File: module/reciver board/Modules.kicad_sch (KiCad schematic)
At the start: 25 parts, among them U10 LTC4316xDD, U13 OSMC Module Board, U14 OSMC Module Board, U15 OSMC Module Board, U16 OSMC Module Board, U17 OSMC Module Board, U18 OSMC Module Board, U19 OSMC Module Board, U20 OSMC Module Board, U5 LTC4316xDD, U6 LTC4317

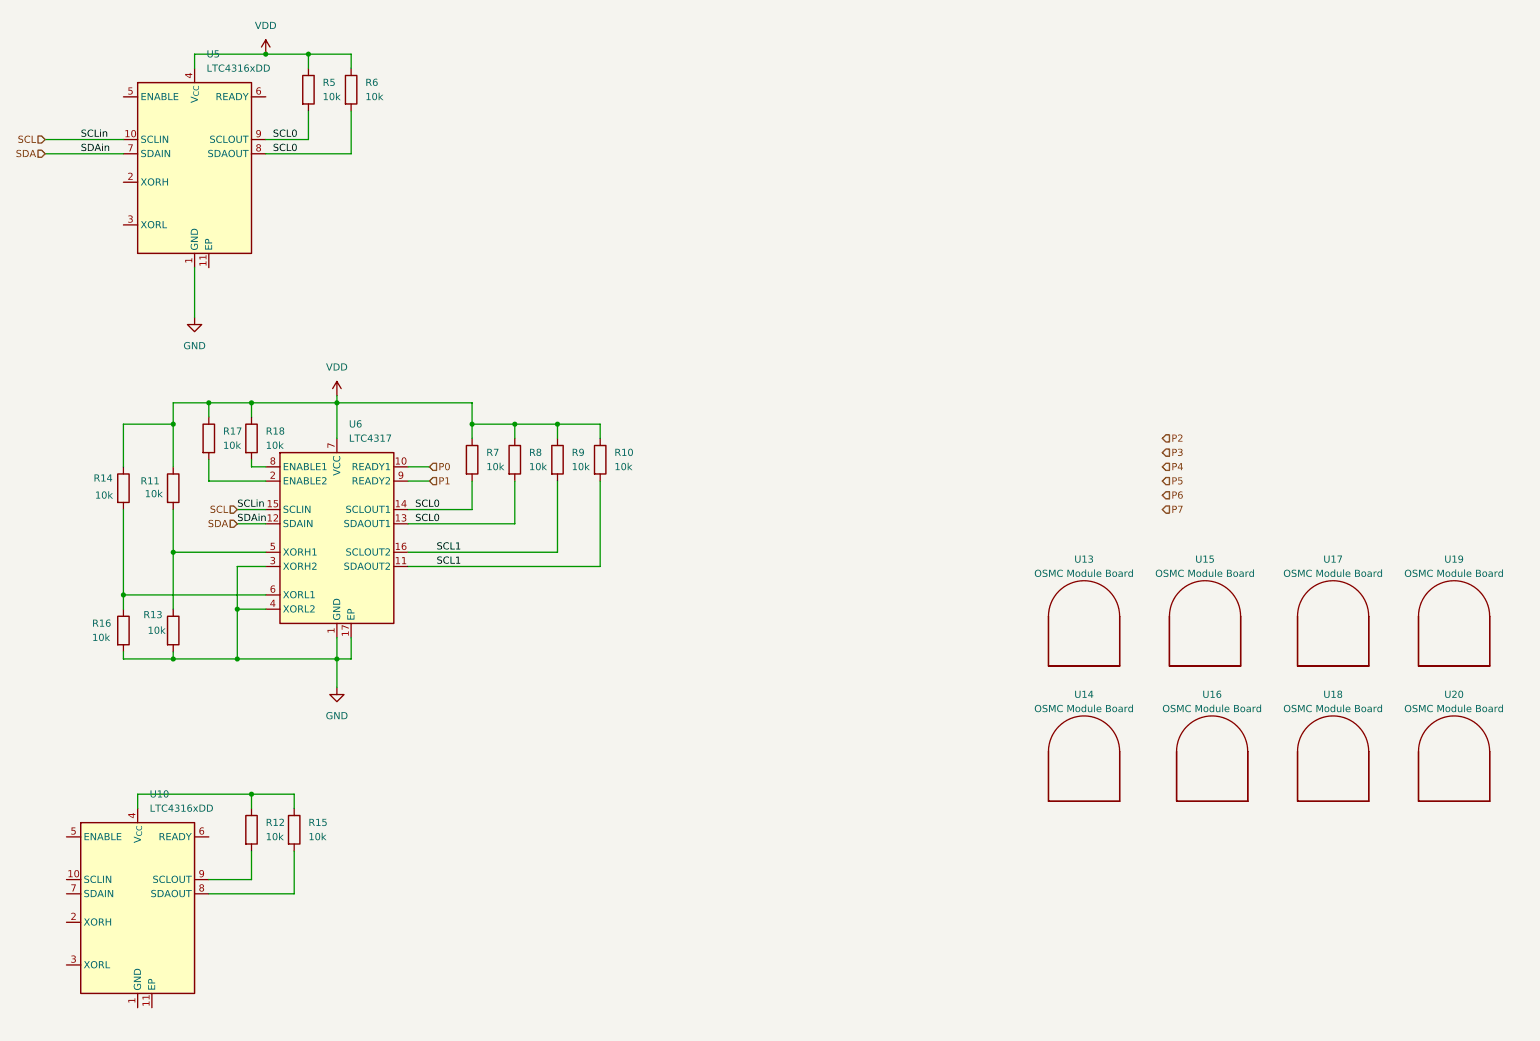
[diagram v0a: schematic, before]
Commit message: update
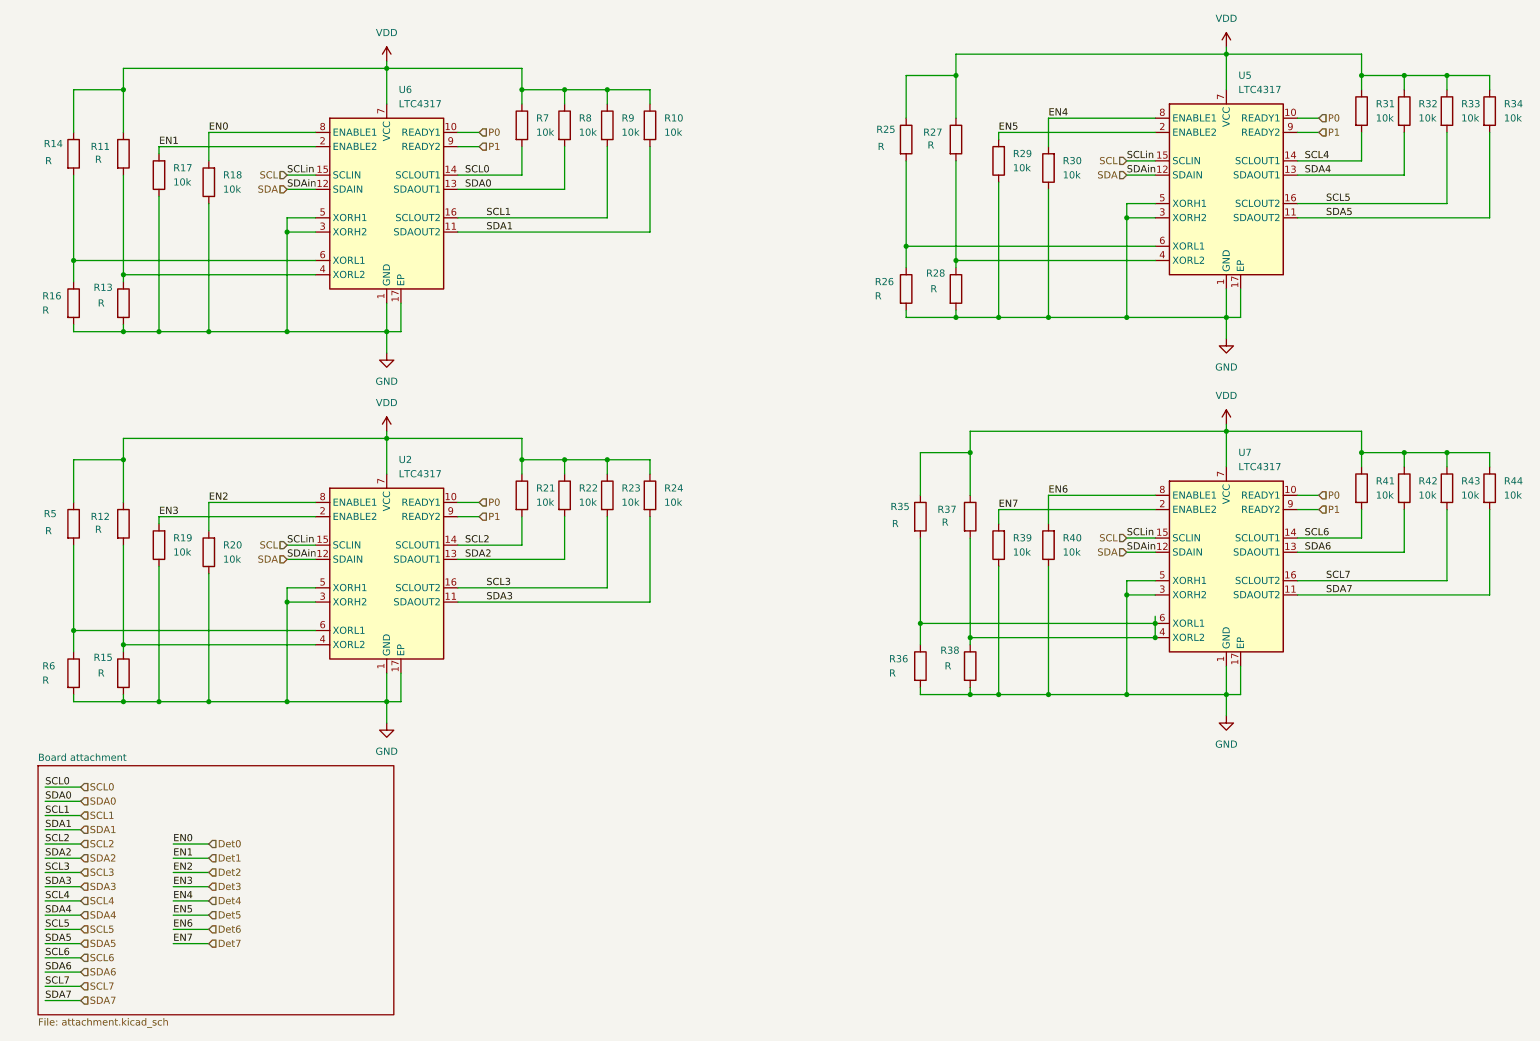
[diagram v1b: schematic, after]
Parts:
- removed U10, U5: LTC4316xDD, Package_DFN_QFN:DFN-10-1EP_3x3mm_P0.5mm_EP1.65x2.38mm, symbol Library:LTC4316xDD
- removed U13, U14, U15, U16, U17, U18, U19, U20: OSMC Module Board, OSMC_Module:Module standard large, symbol Library:Input_Module_Pinless
- added R19, R20, R21, R22, R23, R24, R29, R30, R31, R32, R33, R34, R39, R40, R41, R42, R43, R44: 10k, PCM_Resistor_SMD_AKL:R_0603_1608Metric_Pad1.05x0.95mm_HandSolder, symbol Library:R
- added R25, R26, R27, R28, R35, R36, R37, R38: R, PCM_Resistor_SMD_AKL:R_0603_1608Metric_Pad1.05x0.95mm_HandSolder, symbol Library:R
- added U2, U5, U7: LTC4317, Package_DFN_QFN:DFN-16-1EP_3x5mm_P0.5mm_EP1.66x4.4mm, symbol Library:LTC4317
- R10, R17, R18, R7, R8, R9: footprint PCM_Resistor_SMD_AKL:R_0805_2012Metric_Pad1.15x1.40mm_HandSolder -> PCM_Resistor_SMD_AKL:R_0603_1608Metric_Pad1.05x0.95mm_HandSolder
- R11, R12, R13, R14, R15, R16, R5, R6: value 10k -> R; footprint PCM_Resistor_SMD_AKL:R_0805_2012Metric_Pad1.15x1.40mm_HandSolder -> PCM_Resistor_SMD_AKL:R_0603_1608Metric_Pad1.05x0.95mm_HandSolder
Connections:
- net GND: now also R15.2, R17.1, R18.1, R6.2, U6.5 (XORH1), R19.1, R20.1, R26.2, R28.2, R29.1, R30.1, R36.2, R38.2, R39.1, R40.1, U2.1 (GND), U2.17 (EP), U2.3 (XORH2), U2.5 (XORH1), U5.1 (GND), U5.17 (EP), U5.3 (XORH2), U5.5 (XORH1), U7.1 (GND), U7.17 (EP), U7.3 (XORH2), U7.5 (XORH1); no longer U6.4 (XORL2)
- net P0: now also U2.10 (READY1), U5.10 (READY1), U7.10 (READY1)
- net P1: now also U2.9 (READY2), U5.9 (READY2), U7.9 (READY2)
- net SCL: now also U2.15 (SCLIN), U5.15 (SCLIN), U7.15 (SCLIN)
- net SCL0: no longer R5.2, R6.2, R8.2, U6.13 (SDAOUT1)
- net SCL1: no longer R10.2, U6.11 (SDAOUT2)
- net SDA: now also U2.12 (SDAIN), U5.12 (SDAIN), U7.12 (SDAIN)
- net VDD: now also R12.1, R21.1, R22.1, R23.1, R24.1, R25.1, R27.1, R31.1, R32.1, R33.1, R34.1, R35.1, R37.1, R41.1, R42.1, R43.1, R44.1, U2.7 (VCC), U5.7 (VCC), U7.7 (VCC); no longer R17.1, R18.1, R6.1
- net Det1: now reaches R17.2, U6.2 (ENABLE2)
- net at R11.2, R13.1: now also U6.4 (XORL2); no longer U6.5 (XORH1)
- net Det0: now reaches R18.2, U6.8 (ENABLE1)
- net at R15.1: now also R12.2, U2.4 (XORL2); no longer R12.1
- new net: R35.2, R36.1, R37.2, R38.1, U7.4 (XORL2), U7.6 (XORL1)
- new net: R25.2, R26.1, U5.6 (XORL1)
- new net: R5.2, R6.1, U2.6 (XORL1)
- new net: R27.2, R28.1, U5.4 (XORL2)
- new net Det2: R20.2, U2.8 (ENABLE1)
- new net Det3: R19.2, U2.2 (ENABLE2)
- new net Det4: R30.2, U5.8 (ENABLE1)
- new net Det5: R29.2, U5.2 (ENABLE2)
- new net Det6: R40.2, U7.8 (ENABLE1)
- new net Det7: R39.2, U7.2 (ENABLE2)
- new net SCL2: R21.2, U2.14 (SCLOUT1)
- new net SCL3: R23.2, U2.16 (SCLOUT2)
- new net SCL4: R31.2, U5.14 (SCLOUT1)
- new net SCL5: R33.2, U5.16 (SCLOUT2)
- new net SCL6: R41.2, U7.14 (SCLOUT1)
- new net SCL7: R43.2, U7.16 (SCLOUT2)
- new net SDA0: R8.2, U6.13 (SDAOUT1)
- new net SDA1: R10.2, U6.11 (SDAOUT2)
- new net SDA2: R22.2, U2.13 (SDAOUT1)
- new net SDA3: R24.2, U2.11 (SDAOUT2)
- new net SDA4: R32.2, U5.13 (SDAOUT1)
- new net SDA5: R34.2, U5.11 (SDAOUT2)
- new net SDA6: R42.2, U7.13 (SDAOUT1)
- new net SDA7: R44.2, U7.11 (SDAOUT2)
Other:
- added sheet Board attachment (attachment.kicad_sch)
- moved on the sheet: R10, R11, R13, R14, R16, R17, R18, R7, R8, R9, U6
